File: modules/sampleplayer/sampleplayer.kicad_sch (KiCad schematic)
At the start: 4 parts, among them J1 AudioJack2_SwitchT, U1 ESP32-DEVKIT-V1

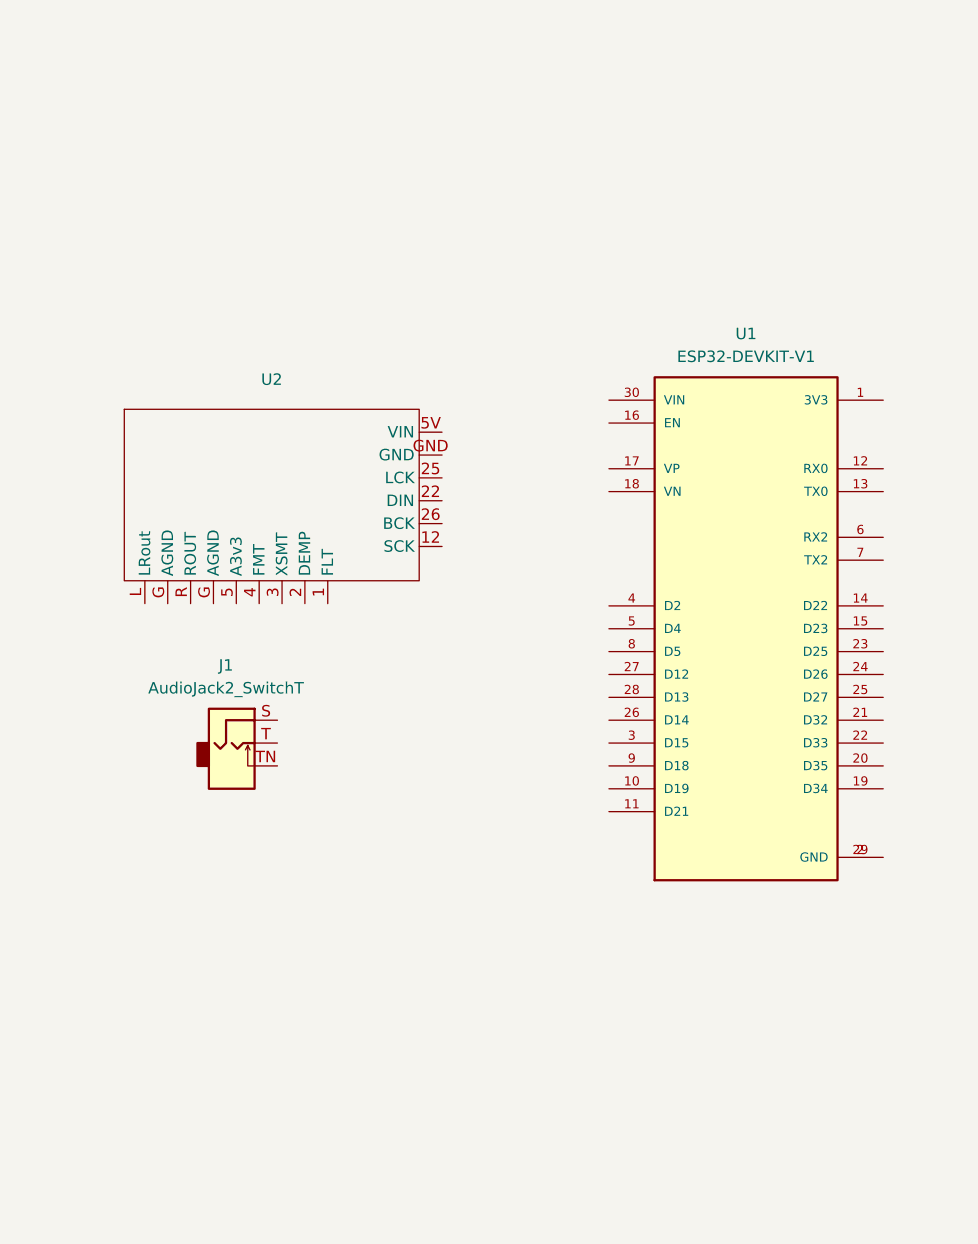
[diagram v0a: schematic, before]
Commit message: upodates
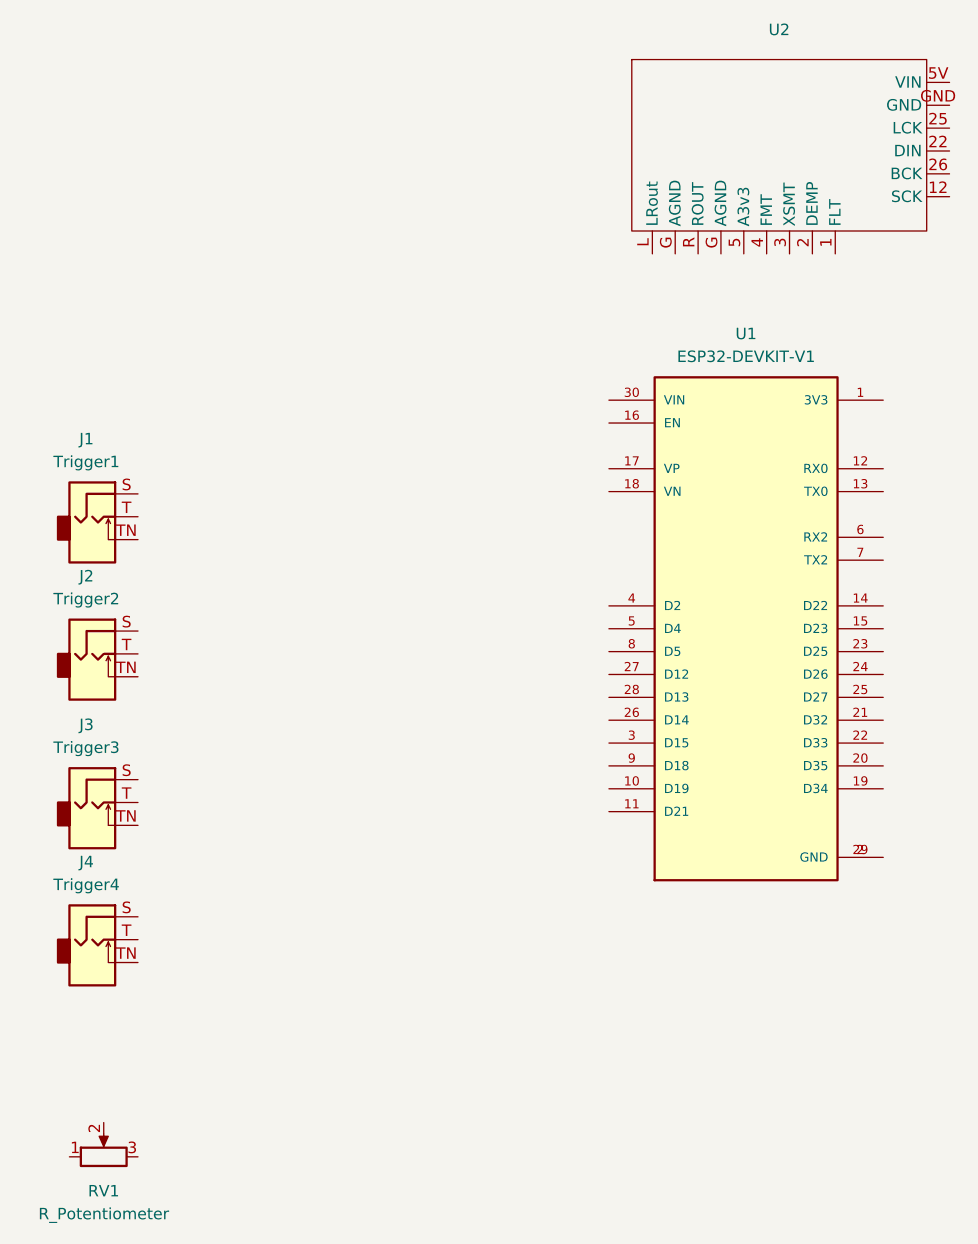
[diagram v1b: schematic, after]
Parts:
- added J2: Trigger2, AudioJacks:Jack_3.5mm_QingPu_WQP-PJ301M-12_Vertical, symbol Connector_Audio:AudioJack2_SwitchT
- added J3: Trigger3, AudioJacks:Jack_3.5mm_QingPu_WQP-PJ301M-12_Vertical, symbol Connector_Audio:AudioJack2_SwitchT
- added J4: Trigger4, AudioJacks:Jack_3.5mm_QingPu_WQP-PJ301M-12_Vertical, symbol Connector_Audio:AudioJack2_SwitchT
- added RV1: R_Potentiometer, symbol Device:R_Potentiometer
- J1: value AudioJack2_SwitchT -> Trigger1
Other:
- moved on the sheet: J1, U2

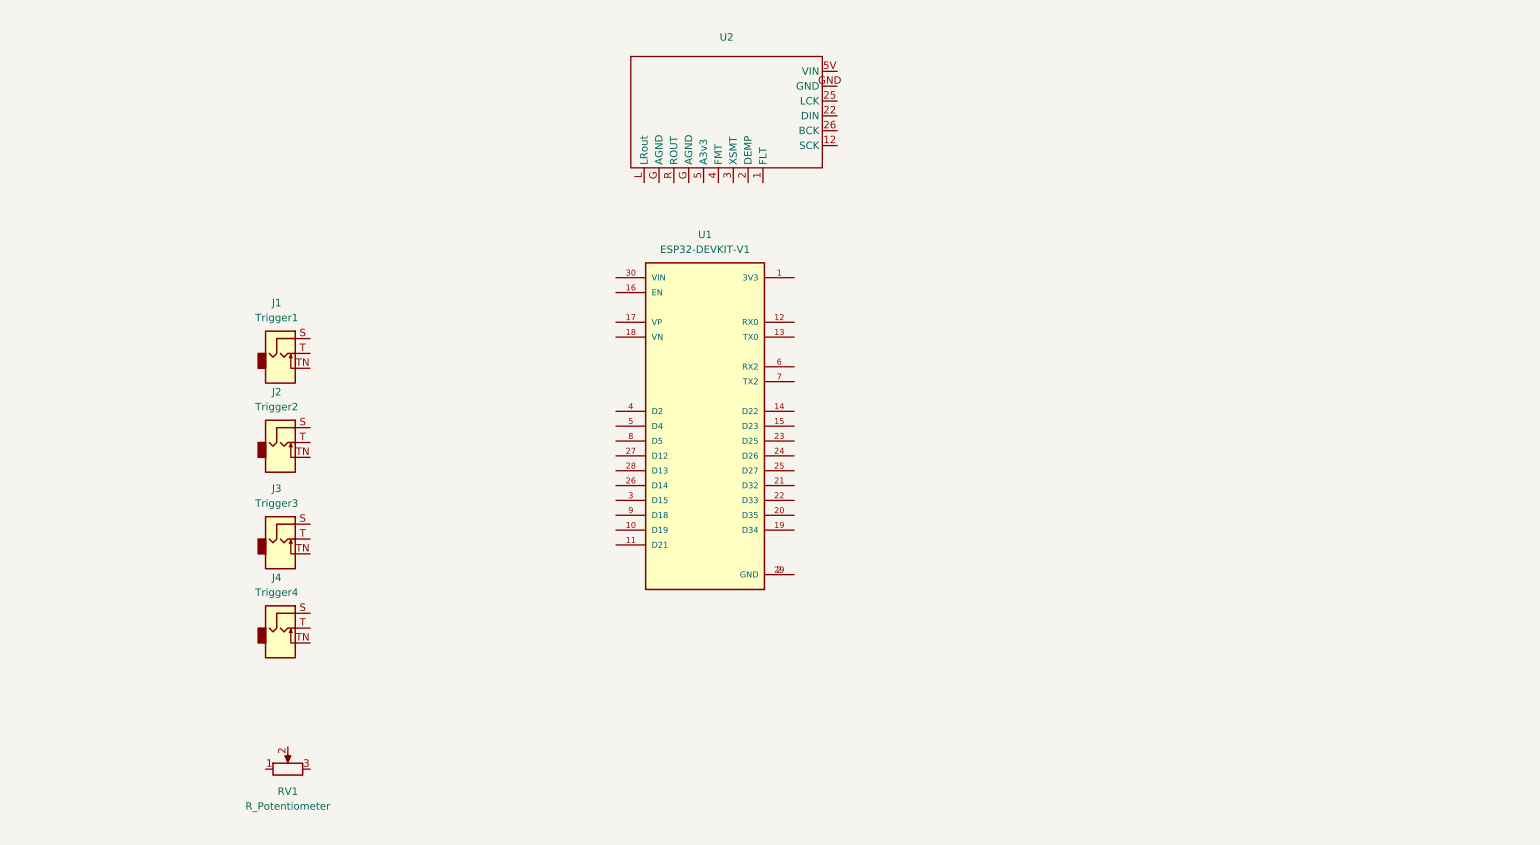
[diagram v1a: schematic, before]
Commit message: sampleplayer update
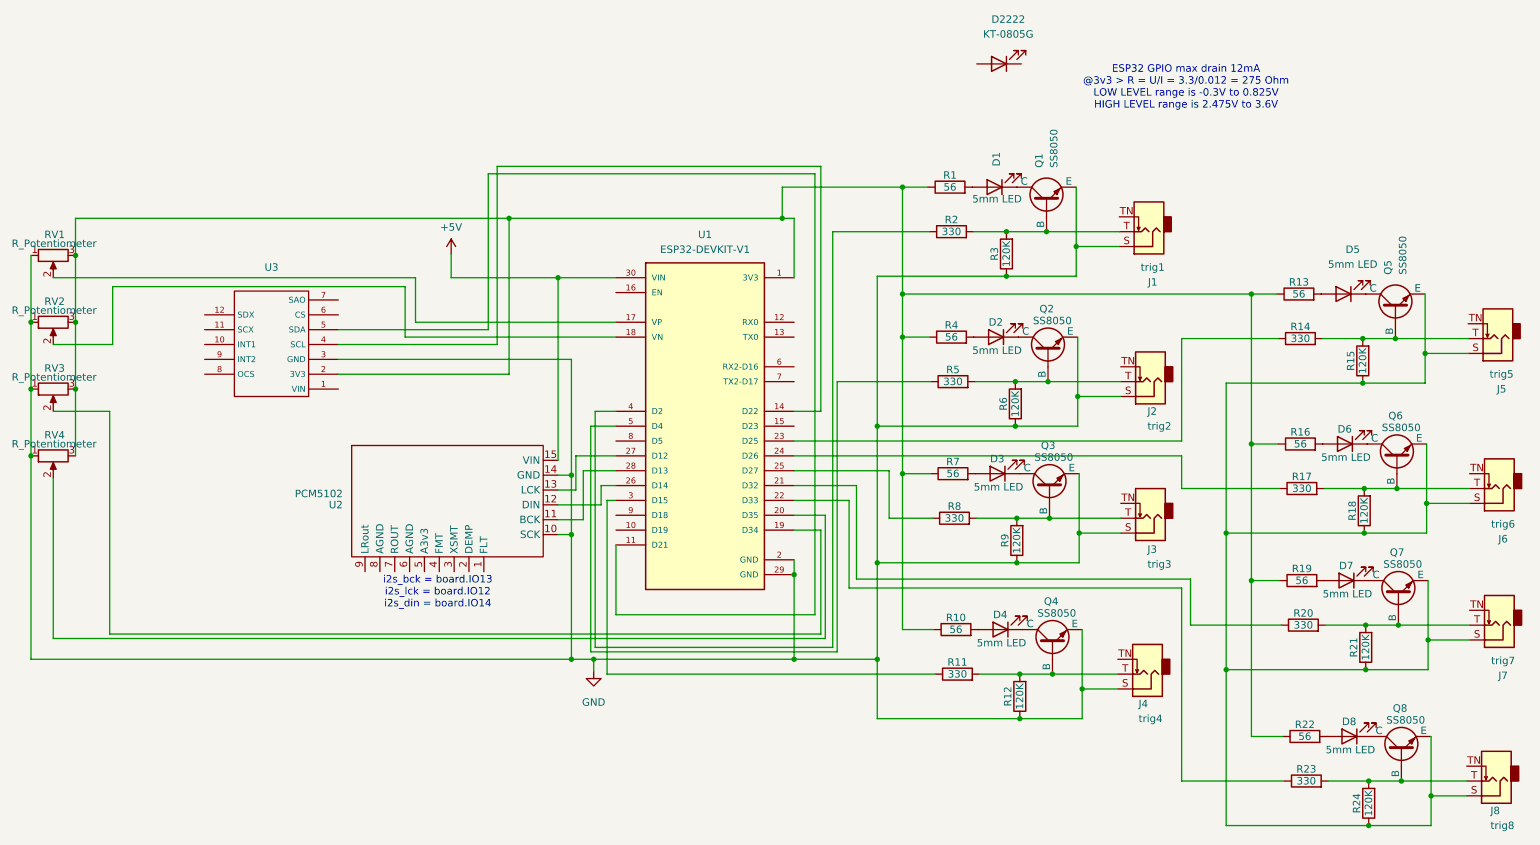
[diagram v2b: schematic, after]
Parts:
- removed ESP32DEV1: ~, symbol ESP32boards:ESP-WROOM-32_30pinboard
- added D1, D2, D3, D4, D5, D6, D7, D8: 5mm LED, LED_THT:LED_D5.0mm, symbol Device:LED
- added D2222: KT-0805G, LED_SMD:LED_0805_2012Metric, symbol Device:LED
- added J5: trig5, AudioJacks:Jack_3.5mm_QingPu_WQP-PJ301M-12_Vertical, symbol Connector_Audio:AudioJack2_SwitchT
- added J6: trig6, AudioJacks:Jack_3.5mm_QingPu_WQP-PJ301M-12_Vertical, symbol Connector_Audio:AudioJack2_SwitchT
- added J7: trig7, AudioJacks:Jack_3.5mm_QingPu_WQP-PJ301M-12_Vertical, symbol Connector_Audio:AudioJack2_SwitchT
- added J8: trig8, AudioJacks:Jack_3.5mm_QingPu_WQP-PJ301M-12_Vertical, symbol Connector_Audio:AudioJack2_SwitchT
- added Q1, Q2, Q3, Q4, Q5, Q6, Q7, Q8: SS8050, Package_TO_SOT_SMD:SOT-23-3, symbol Simulation_SPICE:NPN
- added R1, R10, R13, R16, R19, R22, R4, R7: 56, Resistor_SMD:R_0201_0603Metric, symbol Device:R
- added R11, R14, R17, R2, R20, R23, R5, R8: 330, Resistor_SMD:R_0201_0603Metric, symbol Device:R
- added R12, R15, R18, R21, R24, R3, R6, R9: 120K, Resistor_SMD:R_0201_0603Metric, symbol Device:R
- added RV2, RV3, RV4: R_Potentiometer, Potentiometer_THT:Potentiometer_Alps_RK09K_Single_Vertical, symbol Device:R_Potentiometer
- added U3: ~, breakoutboards:BMI160, symbol breakoutboards:BMI160
- J1: renamed from J4; value Trigger4 -> trig1
- J2: renamed from J3; value Trigger3 -> trig2
- J3: renamed from J2; value Trigger2 -> trig3
- J4: renamed from J1; value Trigger1 -> trig4
- RV1: footprint (none) -> Potentiometer_THT:Potentiometer_Alps_RK09K_Single_Vertical
- U1: symbol ESP32boards:ESP32-DEVKIT-V1 -> ESP32-boards:ESP32-DEVKIT-V1
- U2: value ~ -> PCM5102
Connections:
- net GND: now reaches J3.S
- net GND: now also J1.S, J2.S, J4.S, RV1.1, U1.2 (GND), U1.29 (GND), U2.10 (SCK), U2.14 (GND), Q1.3 (E), Q2.3 (E), Q3.3 (E), Q4.3 (E), R12.1, R3.1, R6.1, R9.1, RV2.1, RV3.1, RV4.1, U3.3 (GND)
- net at J3.T: now also Q3.2 (B), R8.2, R9.2
- net at J1.T: now also Q1.2 (B), R2.2, R3.2
- net at J2.T: now also Q2.2 (B), R5.2, R6.2
- net at U1.1 (3V3): now also RV1.3, R1.1, R10.1, R13.1, R16.1, R19.1, R22.1, R4.1, R7.1, RV2.3, RV3.3, RV4.3, U3.2 (3V3)
- net at U1.11 (D21): now also U3.5 (SDA)
- net at U1.14 (D22): now also U3.4 (SCL)
- net at U1.17 (VP): now also RV1.2
- net at U1.18 (VN): now also RV2.2
- net at U1.19 (D34): now also RV3.2
- net at U1.20 (D35): now also RV4.2
- net at U1.21 (D32): now also R20.1
- net at U1.22 (D33): now also R23.1
- net at U1.23 (D25): now also R14.1
- net at U1.24 (D26): now also R17.1
- net at U1.25 (D27): now also R8.1
- net at U1.26 (D14): now also U2.12 (DIN)
- net at U1.27 (D12): now also U2.13 (LCK)
- net at U1.28 (D13): now also U2.11 (BCK)
- net at U1.3 (D15): now also R11.1
- net +5V: now reaches U1.30 (VIN)
- net +5V: now also U2.15 (VIN)
- net at U1.4 (D2): now also R2.1
- net at U1.5 (D4): now also R5.1
- net at J4.T: now also Q4.2 (B), R11.2, R12.2
- new net: D1.1 (K), Q1.1 (C)
- new net: D1.2 (A), R1.2
- new net: D8.1 (K), Q8.1 (C)
- new net: D8.2 (A), R22.2
- new net: D5.1 (K), Q5.1 (C)
- new net: D5.2 (A), R13.2
- new net: J5.T, Q5.2 (B), R14.2, R15.2
- new net: J5.S, J6.S, J7.S, J8.S, Q5.3 (E), Q6.3 (E), Q7.3 (E), Q8.3 (E), R15.1, R18.1, R21.1, R24.1
- new net: J7.T, Q7.2 (B), R20.2, R21.2
- new net: D2.1 (K), Q2.1 (C)
- new net: J8.T, Q8.2 (B), R23.2, R24.2
- new net: D6.2 (A), R16.2
- new net: J6.T, Q6.2 (B), R17.2, R18.2
- new net: D3.1 (K), Q3.1 (C)
- new net: D3.2 (A), R7.2
- new net: D7.2 (A), R19.2
- new net: D2.2 (A), R4.2
- new net: D4.1 (K), Q4.1 (C)
- new net: D7.1 (K), Q7.1 (C)
- new net: D4.2 (A), R10.2
- new net: D6.1 (K), Q6.1 (C)
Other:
- note added: "ESP32 GPIO max drain 12mA @3v3 > R = U/I = 3.3/0.012 = 275 Ohm LOW LEVEL range is -0.3V to 0.825V HIGH LEVEL range is 2.475V to 3.6V"
- note added: "i2s_bck = board.IO13 i2s_lck = board.IO12 i2s_din = board.IO14"
- moved on the sheet: J1, J2, J3, J4, RV1, U2
